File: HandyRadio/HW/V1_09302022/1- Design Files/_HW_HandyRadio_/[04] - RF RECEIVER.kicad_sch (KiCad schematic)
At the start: 39 parts, among them J3 MHDR_2POS_VERT, K1 DPDT_RELAY, Q1 MMUN2215LT1G, U3 EGUARD0502A, U4 SI4735-D60-GU

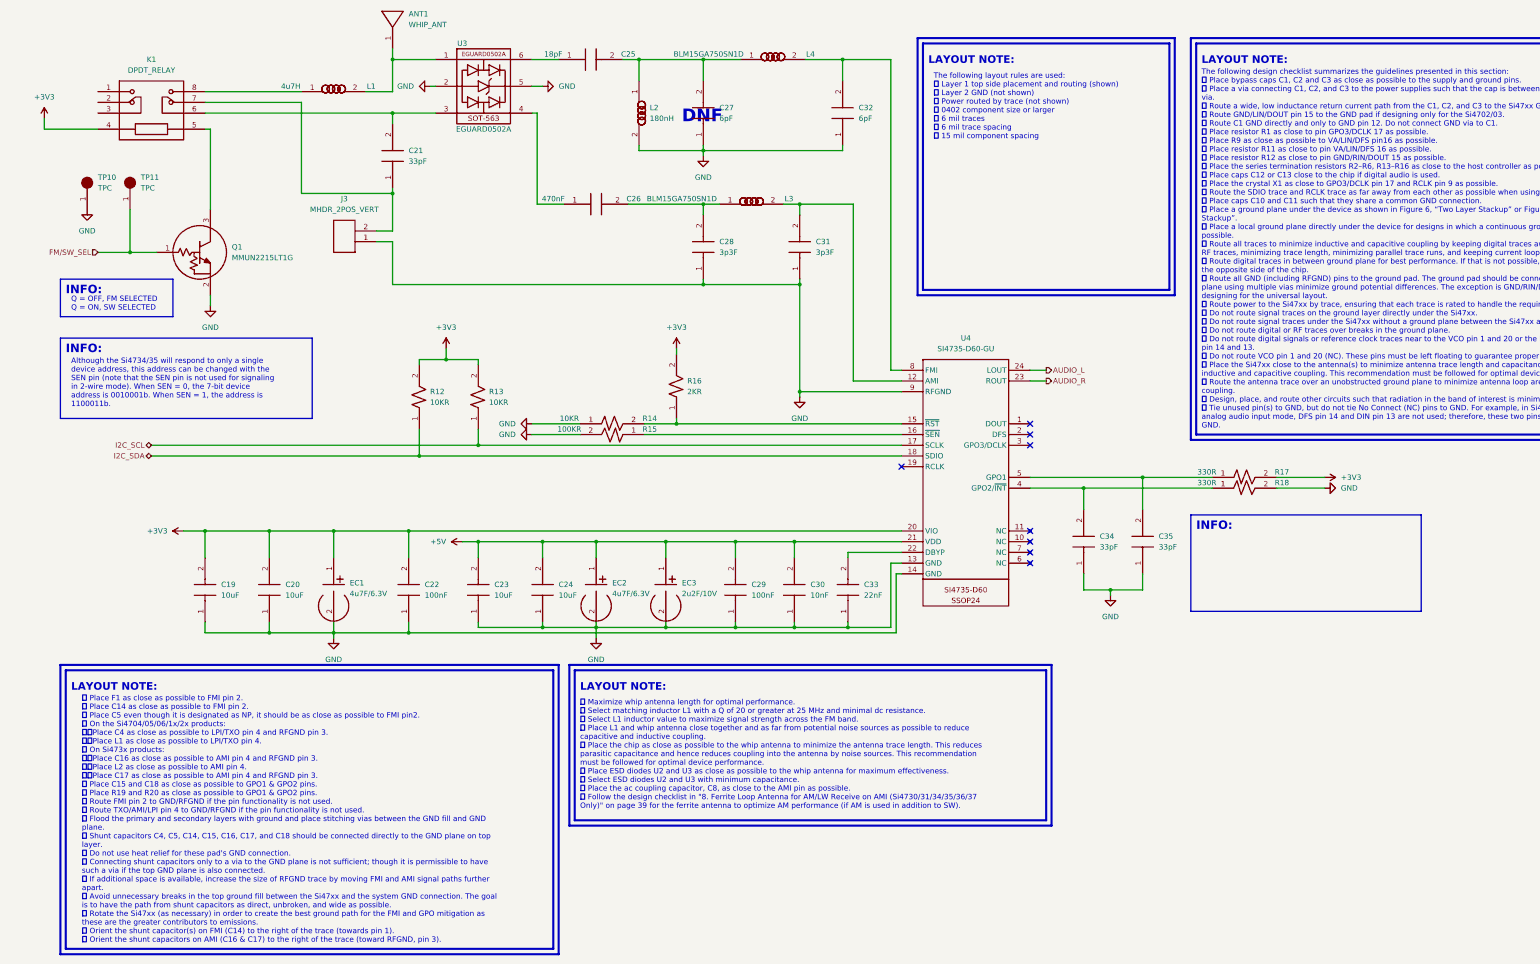
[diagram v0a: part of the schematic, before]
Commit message: Schematic has been double checked
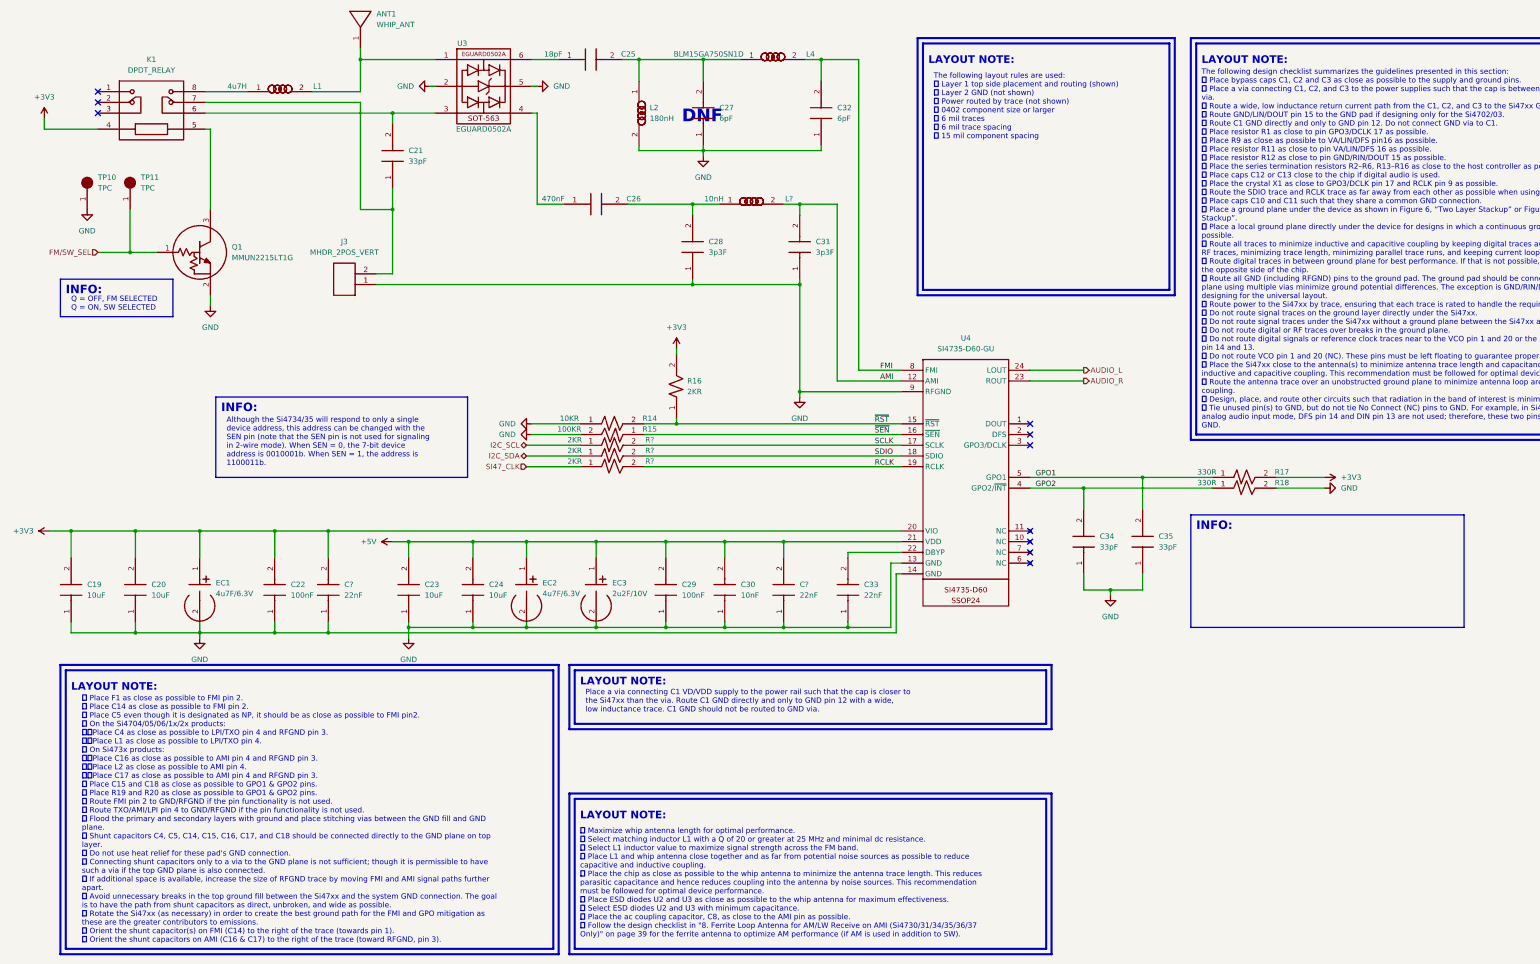
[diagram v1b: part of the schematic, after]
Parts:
- removed L3: BLM15GA750SN1D, symbol HandyRadio:BLM15GA750SN1D
- removed R12, R13: 10KR, symbol HandyRadio:10KR
- added C? (x2): 22nF, symbol HandyRadio:22nF
- added L?: 10nH, symbol HandyRadio:10nH
- added R? (x3): 2KR, symbol HandyRadio:2KR
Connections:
- net +3V3: now also C?.2
- net +5V: now also C?.2
- net GND: now also C?.1, C?.1
- net I2C_SCL: now also R?.1; no longer U4.17 (SCLK)
- net I2C_SDA: now also R?.1; no longer U4.18 (SDIO)
- net ~{RST}: now reaches R14.2, R16.1, U4.15 (~{RST})
- net GPO2: now reaches C34.2, R18.1, U4.4 (GPO2/~{INT})
- net GPO1: now reaches C35.2, R17.1, U4.5 (GPO1)
- net FMI: now reaches C32.2, L4.2, U4.8 (FMI)
- net at C26.2, C28.2: now also L?.1
- net ~{SEN}: now reaches R15.1, U4.16 (~{SEN})
- net AMI: now reaches C31.2, U4.12 (AMI)
- net AMI: now also L?.2
- net RCLK: now reaches U4.19 (RCLK)
- net RCLK: now also R?.2
- new net SCLK: R?.2, U4.17 (SCLK)
- new net SDIO: R?.2, U4.18 (SDIO)
- new net SI47_CLK: R?.1
- no-connect marks 8 -> 10
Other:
- note added: "Place a via connecting C1 VD/VDD supply to the power rail such that the cap is closer to the Si47xx than the via. Route C1 GND directly and only to GND pin 12 with a wide, low inductance trace. C1 GND should not be routed to GND via."
- moved on the sheet: ANT1, C19, C20, C22, C23, C24, C28, C29, C30, C32, EC1, EC2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
